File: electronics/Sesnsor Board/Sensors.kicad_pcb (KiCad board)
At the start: 2 copper layers, 92 x 88 mm, 19 parts, among them J1 GY-91, J2 JTAG, J3 UART, SW1 SW_Push, SW2 SW_Push, U1 ESP32-WROOM-E, U2 H3LIS100DLTR, Y1 32.768

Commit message: Batter Board almost finished
TODO
- Change mosfets&shunt resistor to new choice
- Adjust inductor for higher voltage
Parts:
- Board1: footprint IMU:Rocket_Layout -> Bluesat:Rocket_Layout
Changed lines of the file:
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@@
     )
   )
-  (footprint "IMU:Rocket_Layout" (layer "F.Cu")
+  (footprint "Bluesat:Rocket_Layout" (layer "F.Cu")
     (at 148.2 80.8)
     (property "Sheetfile" "Sensors.kicad_sch")
@@
       (effects (font (size 1 1) (thickness 0.15)))
     )
-    (fp_line (start -31.81 -24.13) (end -31.81 -25.46) (layer "F.SilkS") (width 0.12))
-    (fp_line (start -31.81 25.46) (end -26.61 25.46) (layer "F.SilkS") (width 0.12))
-    (fp_line (start -26.61 -25.46) (end -26.61 25.46) (layer "F.SilkS") (width 0.12))
-    (fp_line (start -31.81 -22.86) (end -31.81 25.46) (layer "F.SilkS") (width 0.12))
-    (fp_line (start -29.21 -22.86) (end -29.21 -25.46) (layer "F.SilkS") (width 0.12))
     (fp_line (start -29.21 -25.46) (end -26.61 -25.46) (layer "F.SilkS") (width 0.12))
     (fp_line (start -31.81 -22.86) (end -29.21 -22.86) (layer "F.SilkS") (width 0.12))
+    (fp_line (start -26.61 -25.46) (end -26.61 25.46) (layer "F.SilkS") (width 0.12))
+    (fp_line (start -29.21 -22.86) (end -29.21 -25.46) (layer "F.SilkS") (width 0.12))
+    (fp_line (start -31.81 25.46) (end -26.61 25.46) (layer "F.SilkS") (width 0.12))
     (fp_line (start -31.81 -25.46) (end -30.48 -25.46) (layer "F.SilkS") (width 0.12))
+    (fp_line (start -31.81 -22.86) (end -31.81 25.46) (layer "F.SilkS") (width 0.12))
+    (fp_line (start -31.81 -24.13) (end -31.81 -25.46) (layer "F.SilkS") (width 0.12))
+    (fp_line (start -41 41) (end -41 44) (layer "Edge.Cuts") (width 0.12))
+    (fp_line (start -41 44) (end 41 44) (layer "Edge.Cuts") (width 0.12))
+    (fp_line (start -41 -44) (end -41 -41) (layer "Edge.Cuts") (width 0.12))
+    (fp_line (start 41 44) (end 41 41) (layer "Edge.Cuts") (width 0.12))
+    (fp_line (start -46 -41) (end -46 41) (layer "Edge.Cuts") (width 0.12))
     (fp_line (start 46 41) (end 46 -41) (layer "Edge.Cuts") (width 0.12))
+    (fp_line (start 41 -41) (end 41 -44) (layer "Edge.Cuts") (width 0.12))
+    (fp_line (start -46 41) (end -41 41) (layer "Edge.Cuts") (width 0.12))
+    (fp_line (start 46 -41) (end 41 -41) (layer "Edge.Cuts") (width 0.12))
+    (fp_line (start -41 -41) (end -46 -41) (layer "Edge.Cuts") (width 0.12))
     (fp_line (start 41 41) (end 46 41) (layer "Edge.Cuts") (width 0.12))
-    (fp_line (start 41 44) (end 41 41) (layer "Edge.Cuts") (width 0.12))
-    (fp_line (start -41 41) (end -41 44) (layer "Edge.Cuts") (width 0.12))
-    (fp_line (start -41 -44) (end -41 -41) (layer "Edge.Cuts") (width 0.12))
-    (fp_line (start 46 -41) (end 41 -41) (layer "Edge.Cuts") (width 0.12))
-    (fp_line (start -41 44) (end 41 44) (layer "Edge.Cuts") (width 0.12))
     (fp_line (start 41 -44) (end -41 -44) (layer "Edge.Cuts") (width 0.12))
-    (fp_line (start -46 41) (end -41 41) (layer "Edge.Cuts") (width 0.12))
-    (fp_line (start 41 -41) (end 41 -44) (layer "Edge.Cuts") (width 0.12))
-    (fp_line (start -46 -41) (end -46 41) (layer "Edge.Cuts") (width 0.12))
-    (fp_line (start -41 -41) (end -46 -41) (layer "Edge.Cuts") (width 0.12))
     (fp_rect (start 38.6 37) (end -39 -38) (layer "Margin") (width 0.12) (fill none))
     (fp_rect (start -33.02 -27.94) (end -25.4 27.94) (layer "F.CrtYd") (width 0.12) (fill none))
+    (fp_line (start -26.67 -25.4) (end -26.67 25.4) (layer "F.Fab") (width 0.1))
+    (fp_line (start -31.75 25.4) (end -31.75 -24.13) (layer "F.Fab") (width 0.1))
+    (fp_line (start -31.75 -24.13) (end -30.48 -25.4) (layer "F.Fab") (width 0.1))
     (fp_line (start -30.48 -25.4) (end -26.67 -25.4) (layer "F.Fab") (width 0.1))
     (fp_line (start -26.67 25.4) (end -31.75 25.4) (layer "F.Fab") (width 0.1))
-    (fp_line (start -31.75 25.4) (end -31.75 -24.13) (layer "F.Fab") (width 0.1))
-    (fp_line (start -26.67 -25.4) (end -26.67 25.4) (layer "F.Fab") (width 0.1))
-    (fp_line (start -31.75 -24.13) (end -30.48 -25.4) (layer "F.Fab") (width 0.1))
     (pad "" np_thru_hole circle (at -42 0) (size 2 2) (drill 3.2) (layers *.Mask))
-    (pad "" np_thru_hole circle (at 43 0) (size 2 2) (drill 3.2) (layers *.Mask))
     (pad "" np_thru_hole circle (at 0 41) (size 2 2) (drill 3.2) (layers *.Mask))
     (pad "" np_thru_hole circle (at 0 -41) (size 2 2) (drill 3.2) (layers *.Mask))
+    (pad "" np_thru_hole circle (at 43 0) (size 2 2) (drill 3.2) (layers *.Mask))
     (pad "1" thru_hole circle (at -30.48 -24.13) (size 1.7 1.7) (drill 1) (layers *.Cu *.Mask)
       (net 45 "+5V") (pinfunction "5V") (pintype "passive"))

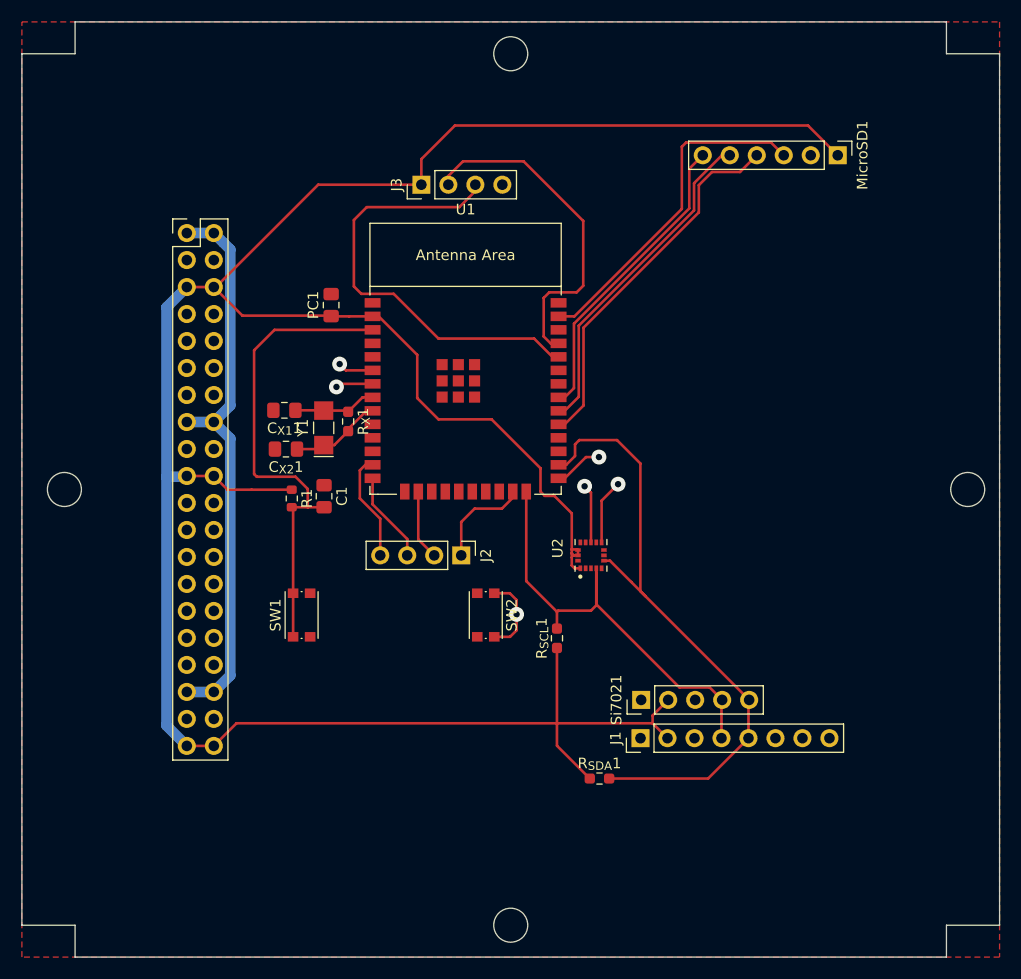
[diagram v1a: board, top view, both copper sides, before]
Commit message: Long overdue commit
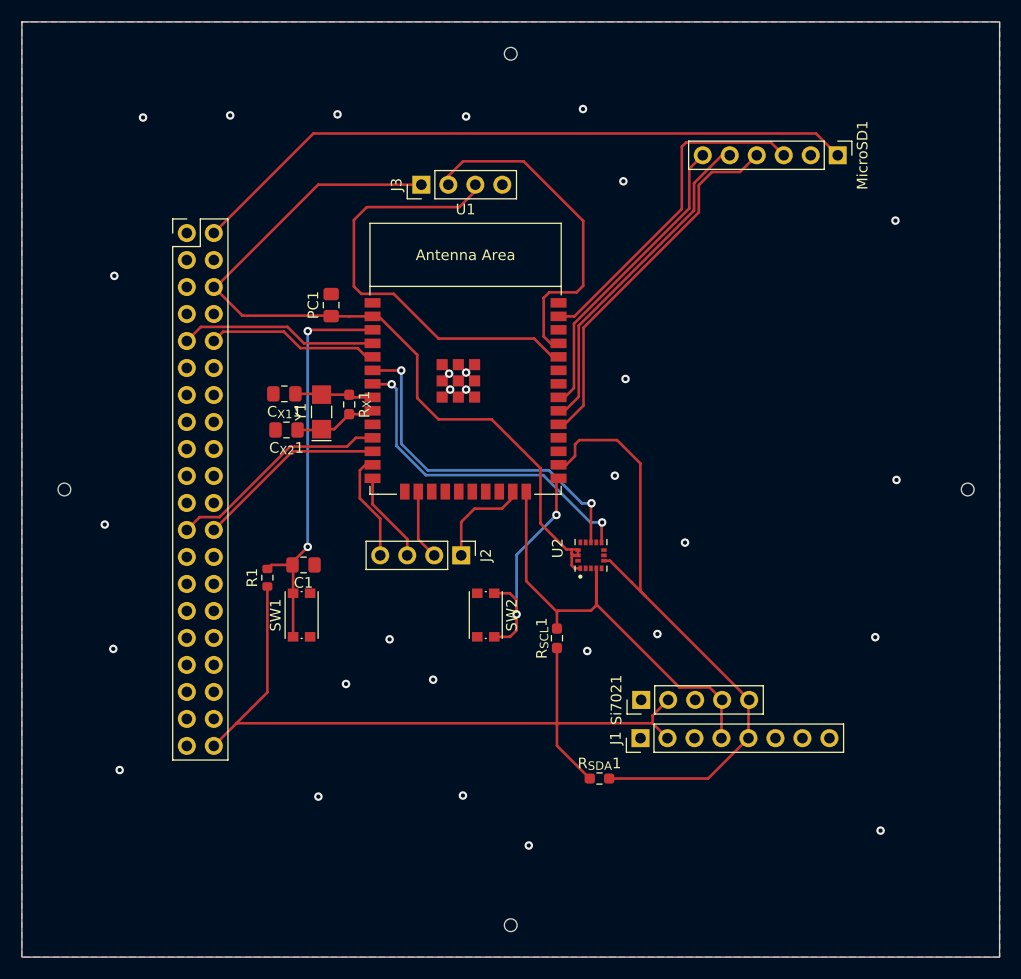
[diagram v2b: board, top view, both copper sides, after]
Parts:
- Board1: footprint Bluesat:Rocket_Layout -> IMU:Rocket_Layout
- moved R1 7.80 mm to (125.3, 89.1), turned to 90 degrees
- moved C1 6.75 mm to (128.7, 87.9), turned to 180 degrees
- moved C_{X2}1 1.80 mm to (127.1, 75.2)
- moved R_{X}1 1.60 mm to (133.0, 72.8)
- moved C_{X1}1 1.55 mm to (126.9, 71.8)
- moved Y1 1.51 mm to (130.4, 73.5)
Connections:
- Board1 pad 12: unconnected-(Board1-Pad12) -> /IO26
- Board1 pad 29: unconnected-(Board1-Pad29) -> /IO27
- Board1 pad 36: unconnected-(Board1-Pad36) -> /I39
- Board1 pad 5: unconnected-(Board1-Pad5) -> /I36
- MicroSD1 pad 1: +3V3 -> +5V
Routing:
- net +3V3: track 244.1 -> 151.7 mm
- net /I34: track 8.87 -> 33.5 mm
- net /I35: track 9.64 -> 32.0 mm
- net /IO26: track 0.00 -> 21.1 mm
- net /I36: track 0.00 -> 18.7 mm
- net /IO27: track 0.00 -> 18.0 mm
- net /I39: track 0.00 -> 16.3 mm
- net +5V: track 53.4 -> 63.4 mm
- net /IO0: track 12.2 -> 22.0 mm
- net Net-(C1-Pad2): track 46.2 -> 38.1 mm, vias 0 -> 2
- net /IO33: track 8.72 -> 7.81 mm
- net GND: vias 0 -> 29
- added copper zone on B.Cu, net GND
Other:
- outline, holes or cut-outs redrawn
